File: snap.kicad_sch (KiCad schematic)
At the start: 29 parts, among them J1 Conn_02x07_Odd_Even, SW1 SW_DPST, SW2 SW_DPST, U1 STM32H7B3VITx, Y1 8kHz, Y2 32.768kHz

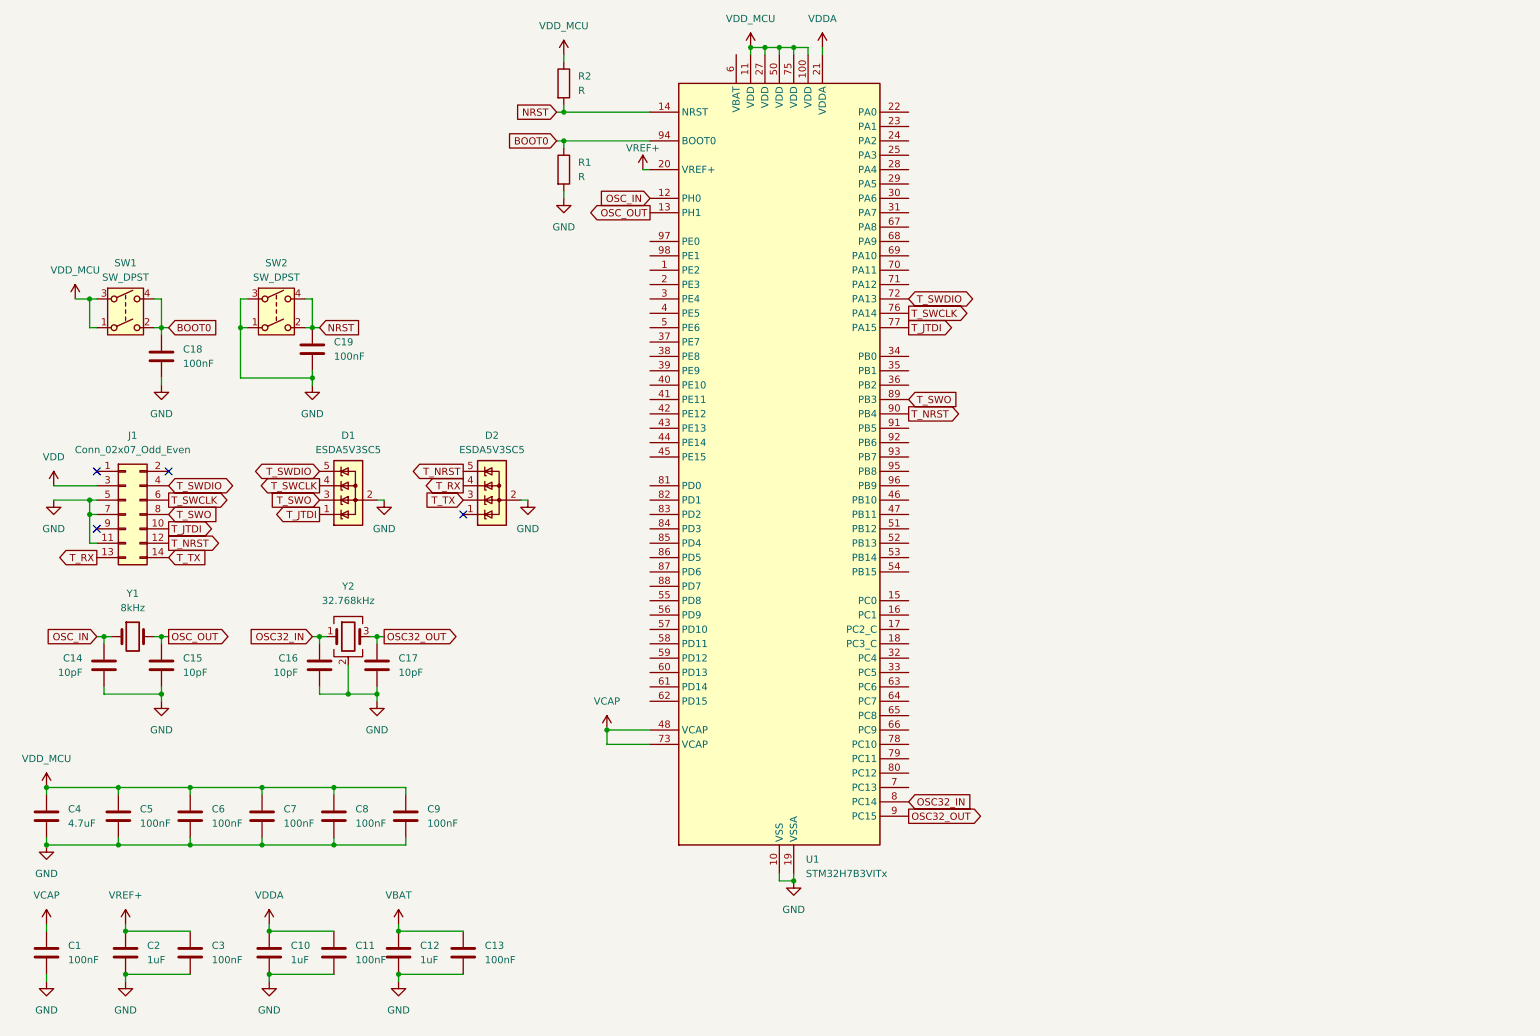
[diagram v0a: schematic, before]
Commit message: actually starting to do the schematics pt.5
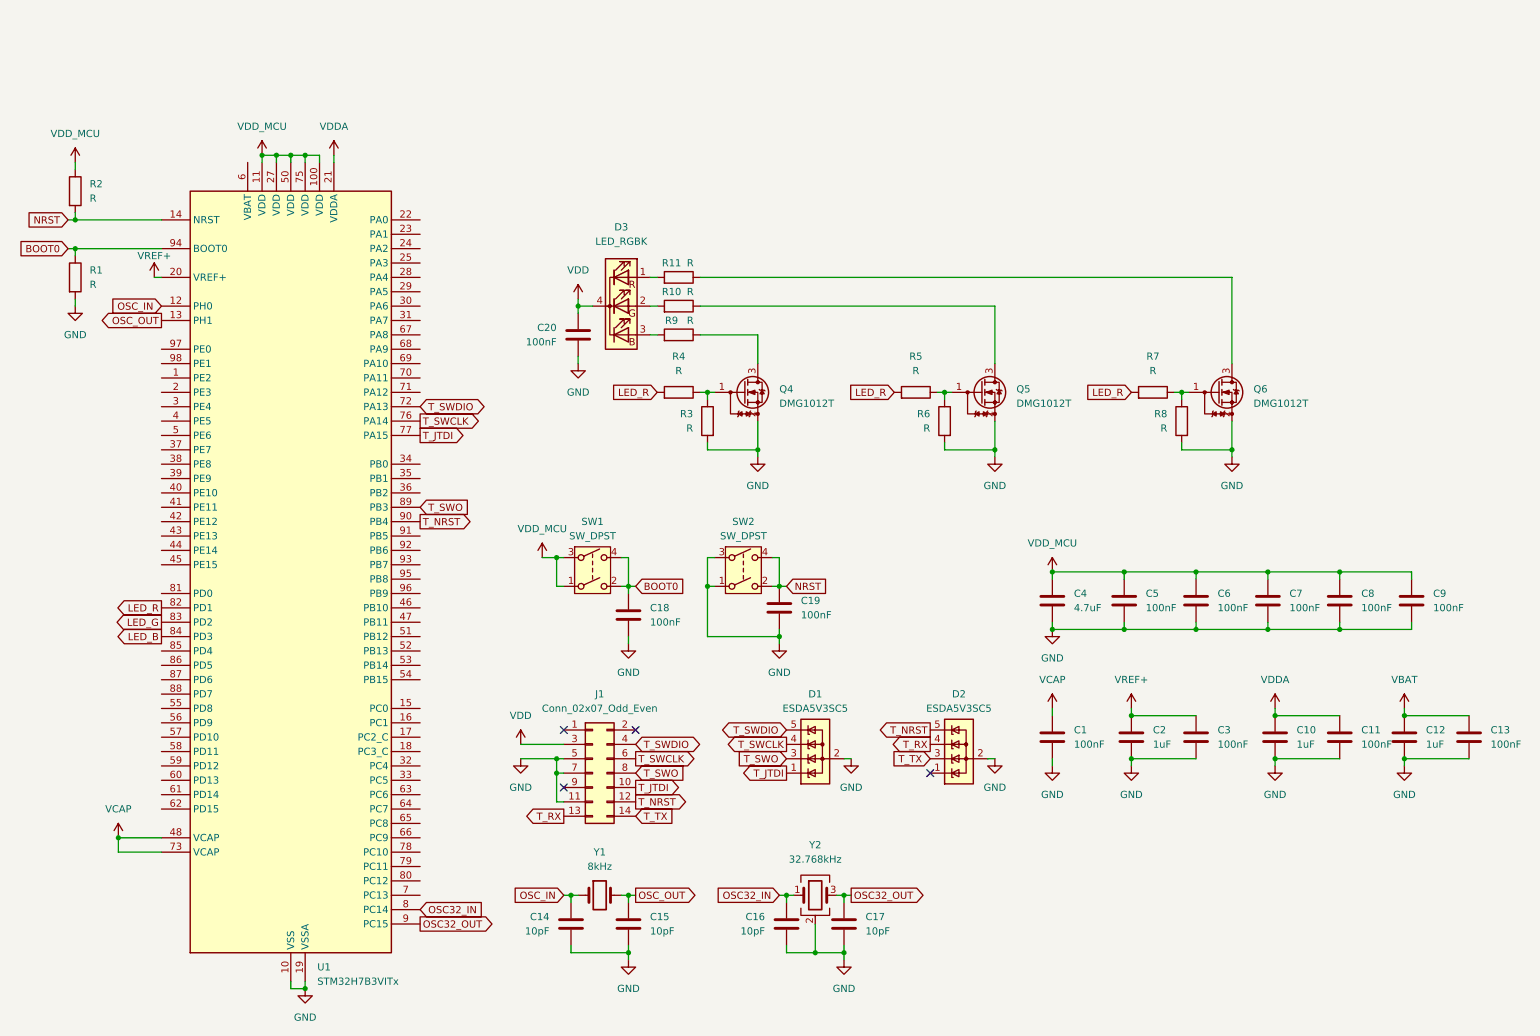
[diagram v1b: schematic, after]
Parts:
- added C20: 100nF, symbol Device:C
- added D3: LED_RGBK, symbol Device:LED_RGBK
- added Q4, Q5, Q6: DMG1012T, Package_TO_SOT_SMD:SOT-523, symbol Transistor_FET:DMG1012T
- added R10, R11, R3, R4, R5, R6, R7, R8, R9: R, symbol Device:R
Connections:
- net GND: now also C20.2, Q4.2 (S), Q5.2 (S), Q6.2 (S), R3.2, R6.2, R8.2
- net VDD: now also C20.1, D3.4 (K)
- net LED_R: now reaches U1.82 (PD1)
- net LED_R: now also R4.2, R5.2, R7.2
- net LED_G: now reaches U1.83 (PD2)
- net LED_B: now reaches U1.84 (PD3)
- new net: Q6.1 (G), R7.1, R8.1
- new net: Q6.3 (D), R11.1
- new net: Q5.1 (G), R5.1, R6.1
- new net: Q5.3 (D), R10.1
- new net: D3.1 (RA), R11.2
- new net: D3.2 (GA), R10.2
- new net: D3.3 (BA), R9.2
- new net: Q4.1 (G), R3.1, R4.1
- new net: Q4.3 (D), R9.1
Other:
- moved on the sheet: C1, C10, C11, C12, C13, C14, C15, C16, C17, C18, C19, C2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
